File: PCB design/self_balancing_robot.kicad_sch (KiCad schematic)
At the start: 31 parts, among them J1 I2C, J2 Analog, J3 left_engine, J4 right_engine, J5 L293D_left, J6 SPI, J7 UART, J8 L293D_right, J9 input_supply, SW1 SW_Push, U1 ATmega328P-A, U4 LP2985-3.3, U5 NCP1117-5.0_SOT223, Y1 Crystal

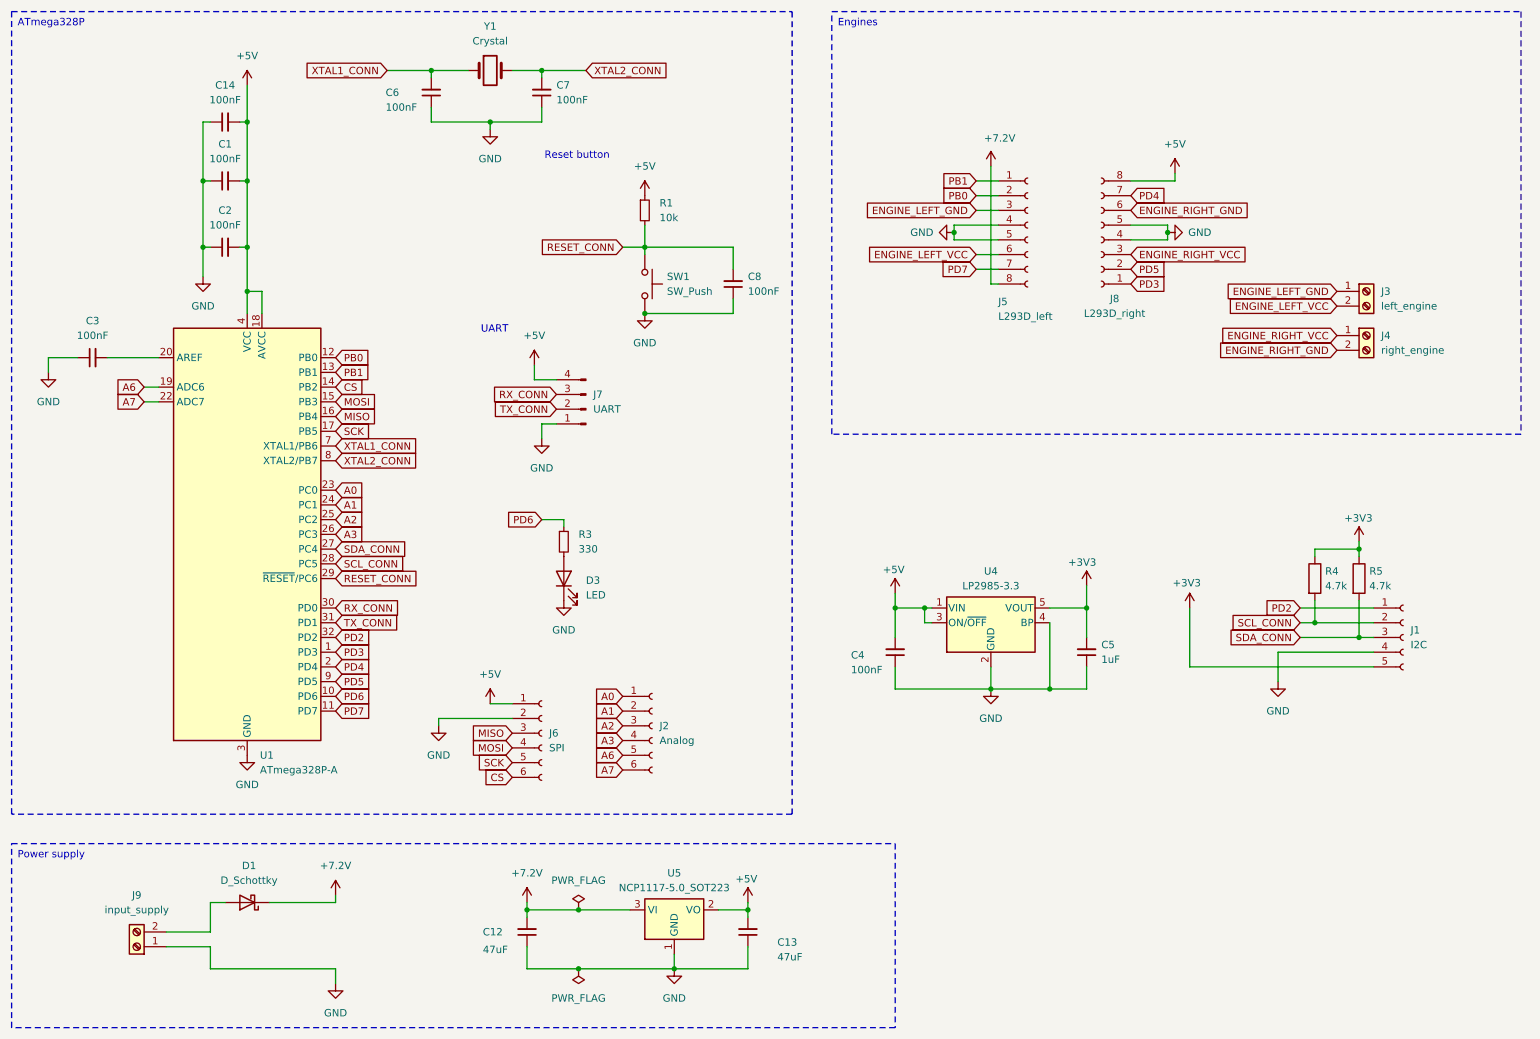
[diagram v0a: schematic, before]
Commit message: PCB update
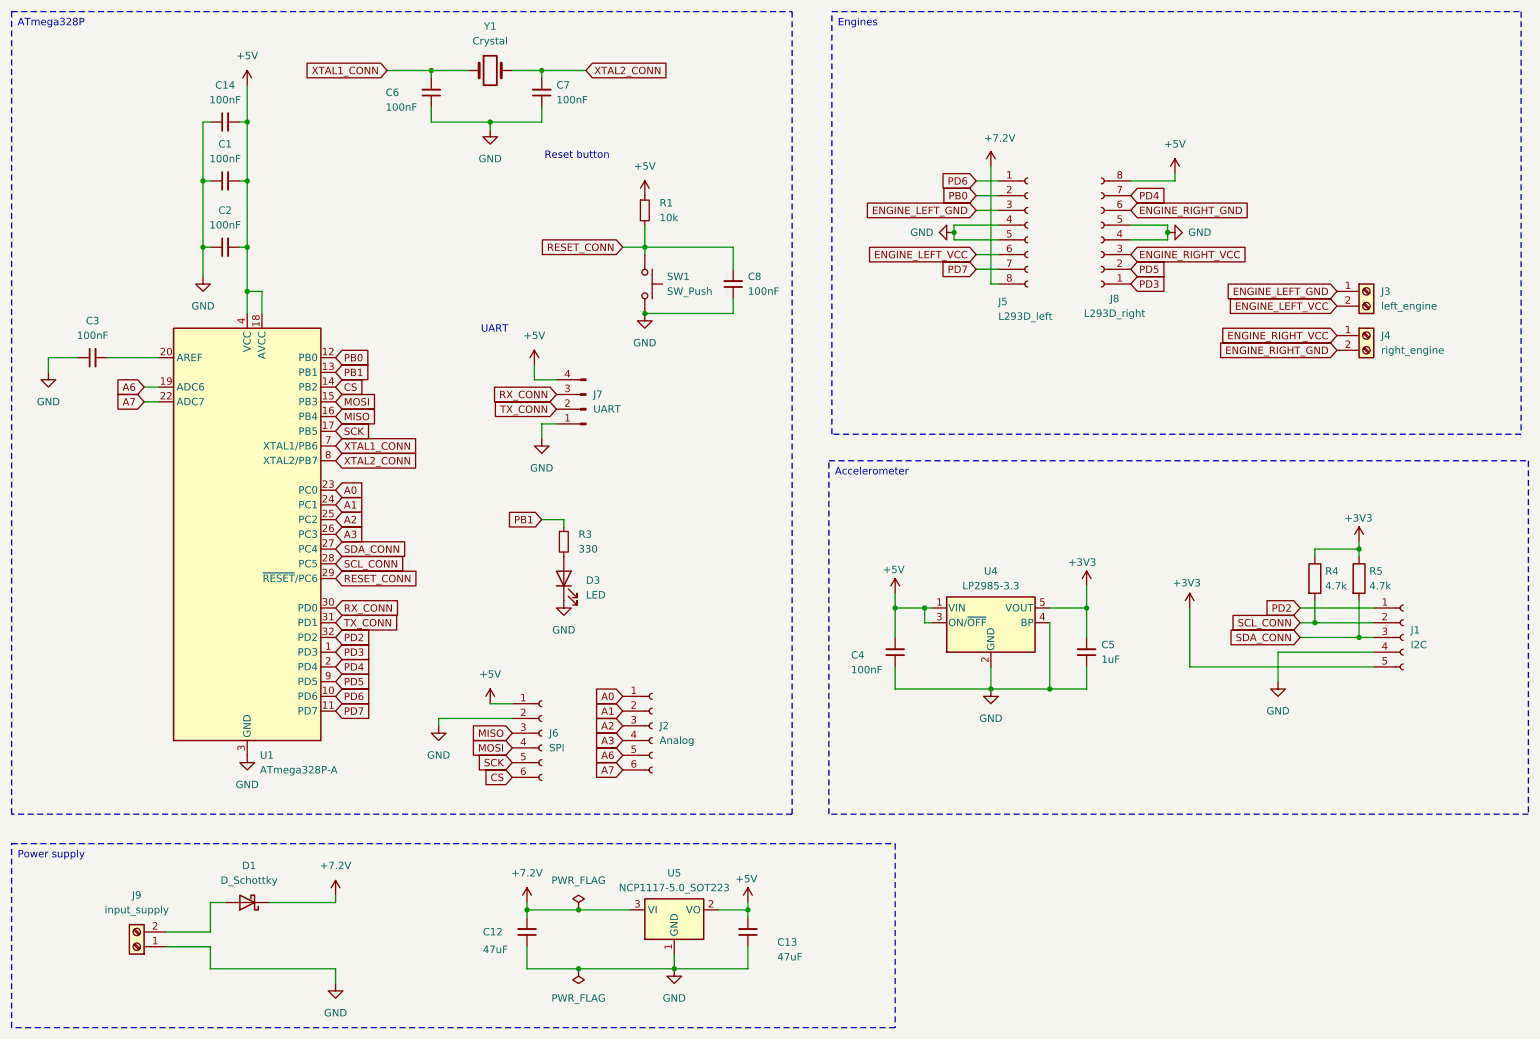
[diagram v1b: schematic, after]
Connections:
- net PB1: now also R3.1; no longer J5.1 (Pin_1)
- net PD6: now also J5.1 (Pin_1); no longer R3.1
